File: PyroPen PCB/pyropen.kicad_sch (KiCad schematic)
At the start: 58 parts, among them J1 AAAA BATT, J2 Front 3.3v LED, J3 MLX90614ESF-DCC-000-TU, J4 BUZZ, J5 DEBUG, SW1 B3U-1000P, U1 ATTINY1616-MNR, U2 MAX17222ELT+T

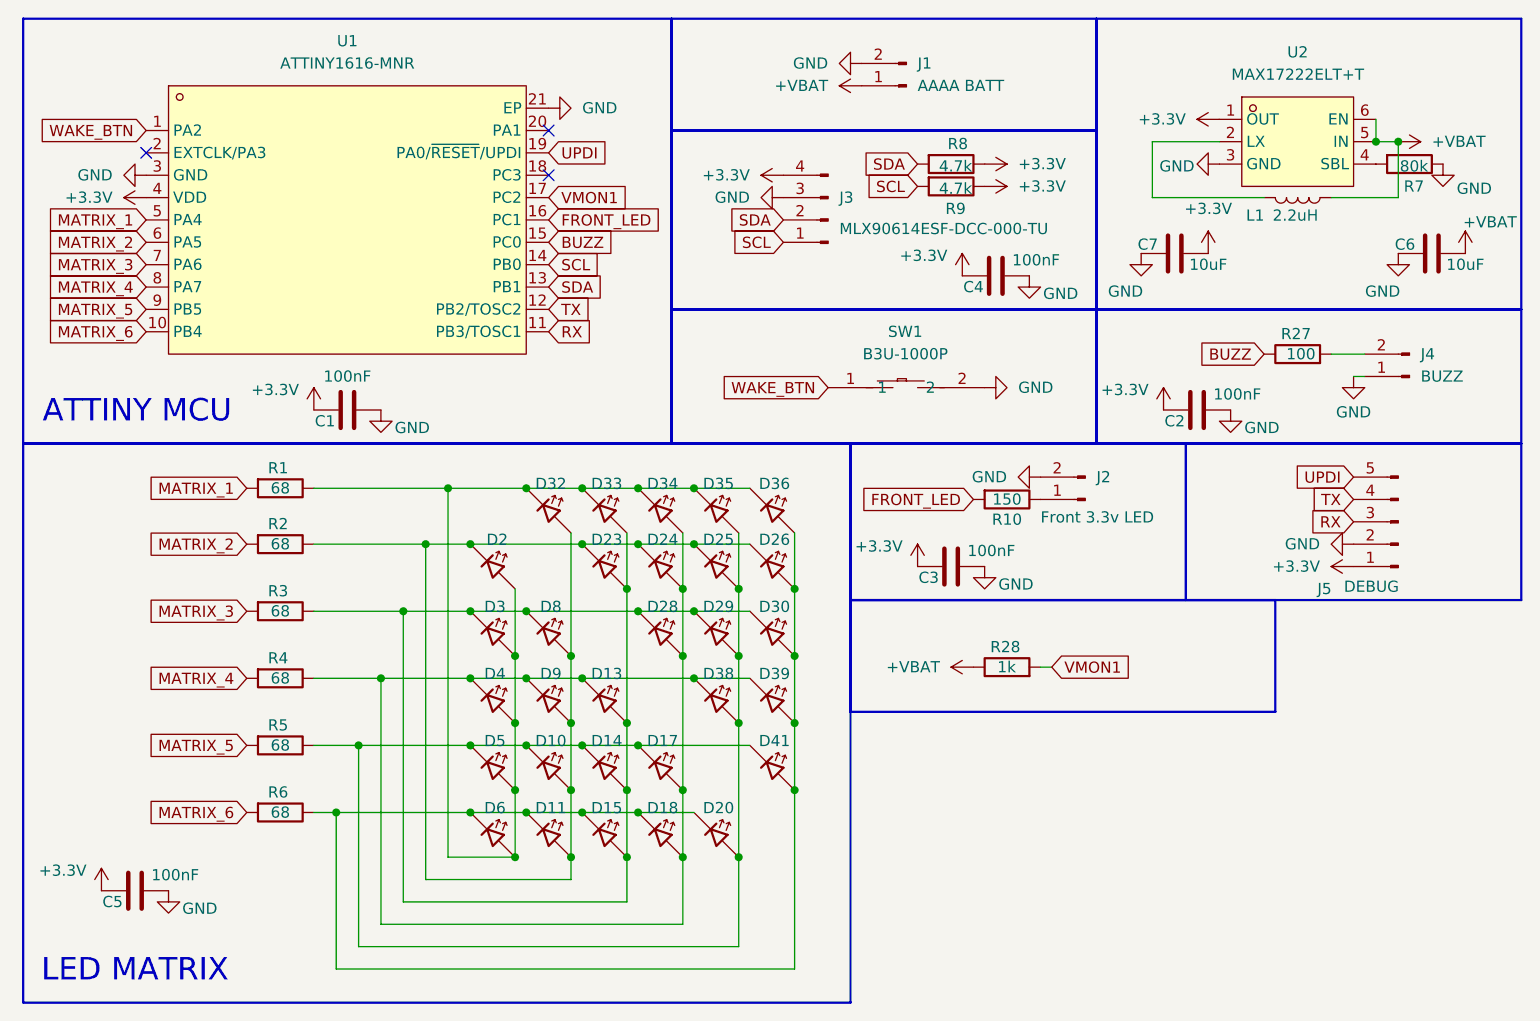
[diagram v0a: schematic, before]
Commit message: sync
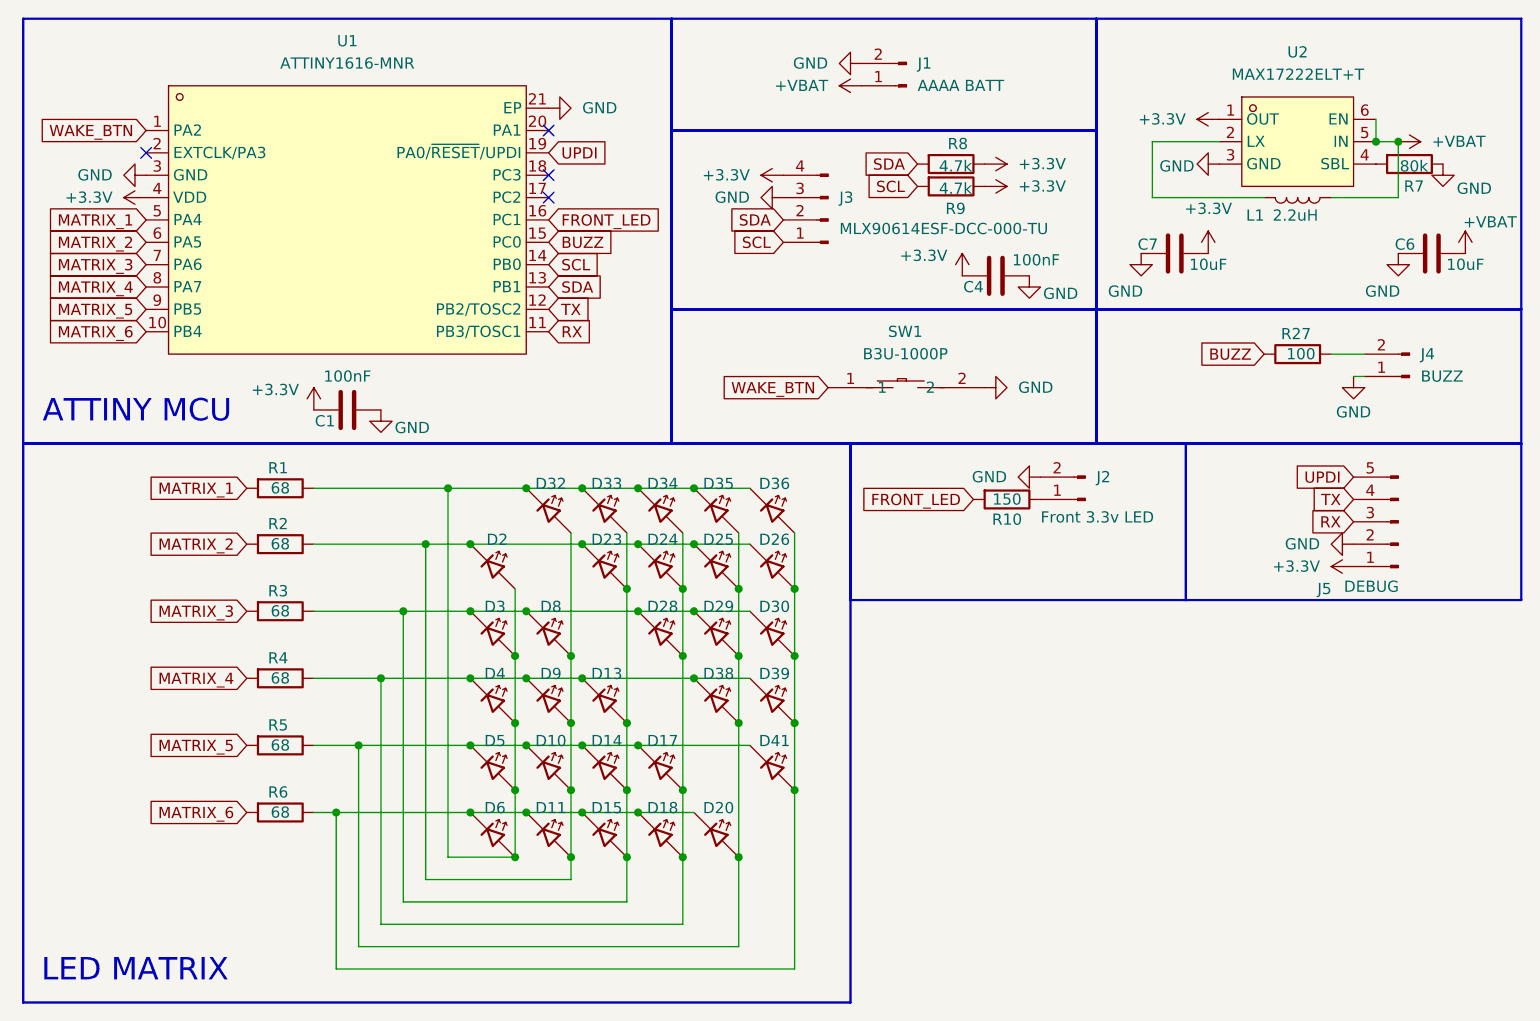
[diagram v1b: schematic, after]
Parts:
- removed C2, C3, C5: 100nF, Capacitor_SMD:C_0402_1005Metric, symbol Device:C
- removed R28: 1k, Resistor_SMD:R_0402_1005Metric, symbol Device:R
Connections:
- net VMON1: no longer names the net of U1.17 (PC2)
- no-connect marks 3 -> 4

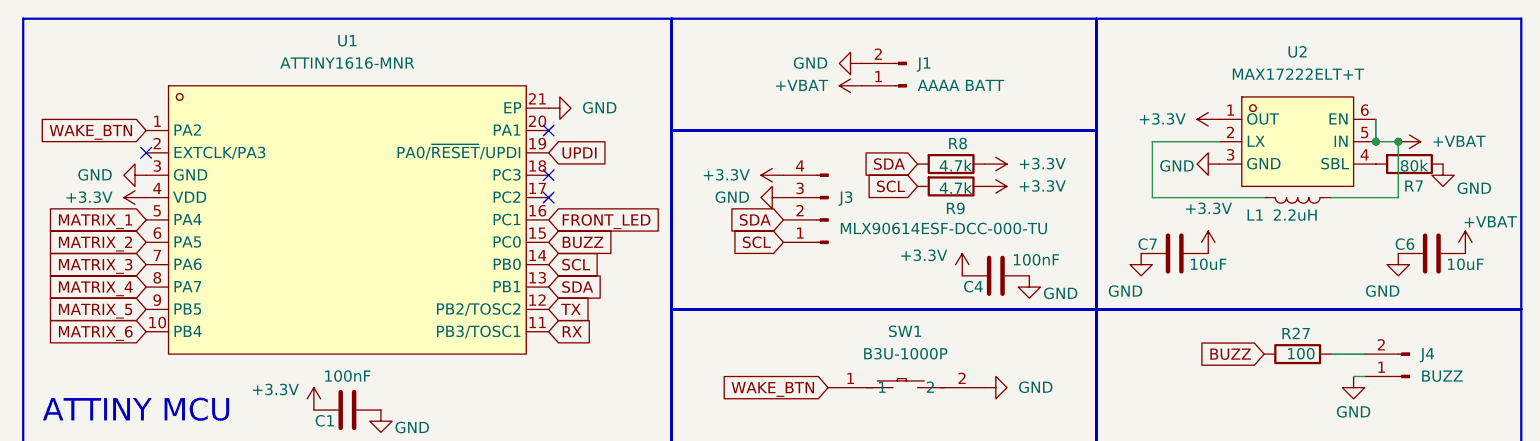
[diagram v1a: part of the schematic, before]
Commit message: sync
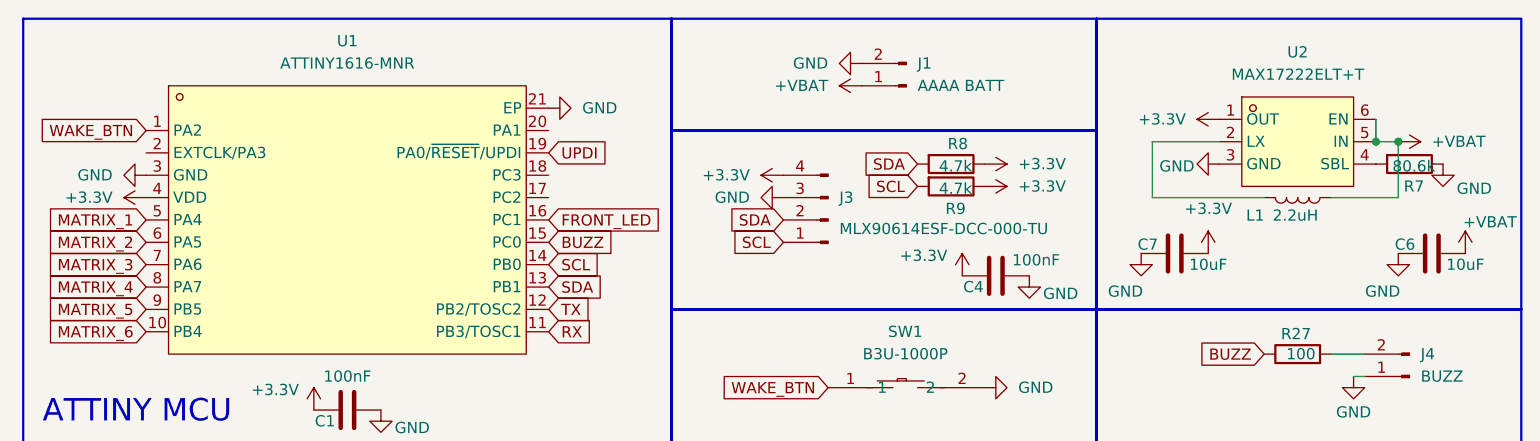
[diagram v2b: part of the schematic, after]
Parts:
- R7: value 80k -> 80.6k
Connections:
- no-connect marks 4 -> 0
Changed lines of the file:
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@@
 		(color 0 0 0 0)
 	)
-	(no_connect
-		(at 74.93 30.48)
-	)
-	(no_connect
-		(at 74.93 25.4)
-	)
-	(no_connect
-		(at 29.21 27.94)
-	)
-	(no_connect
-		(at 74.93 33.02)
-	)
 	(wire
 		(pts
@@
 			)
 		)
-		(property "Value" "80k"
+		(property "Value" "80.6k"
 			(at 173.228 29.464 90)
 			(show_name no)

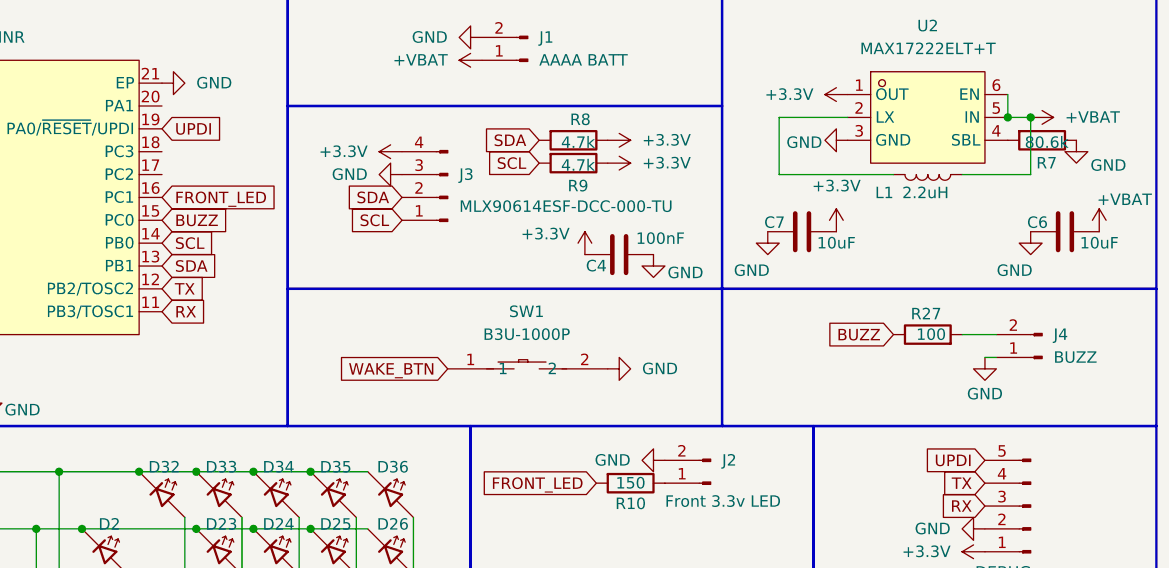
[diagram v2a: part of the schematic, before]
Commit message: sync
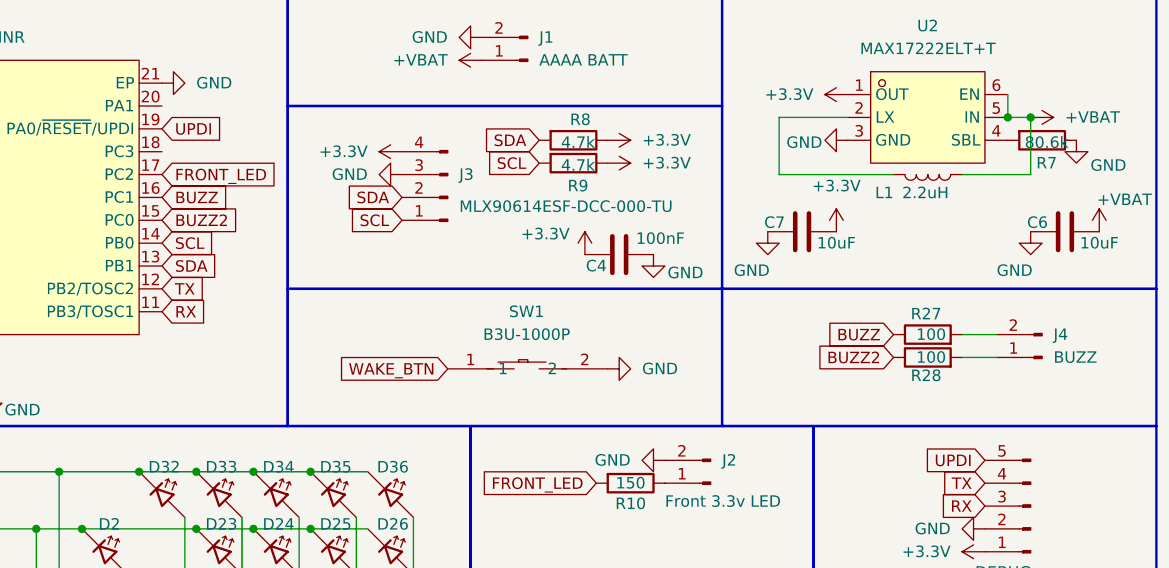
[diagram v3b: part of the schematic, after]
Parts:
- added R28: 100, Resistor_SMD:R_0402_1005Metric, symbol Device:R
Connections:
- net BUZZ: now also U1.16 (PC1); no longer U1.15 (PC0)
- net FRONT_LED: now also U1.17 (PC2); no longer U1.16 (PC1)
- net GND: no longer J4.1 (Pin_1)
- new net: J4.1 (Pin_1), R28.2
- new net BUZZ2: R28.1, U1.15 (PC0)
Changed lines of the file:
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@@
 	(wire
 		(pts
-			(xy 166.37 53.34) (xy 167.64 53.34)
-		)
-		(stroke
-			(width 0)
-			(type default)
-		)
-	)
-	(wire
-		(pts
 			(xy 66.04 80.01) (xy 72.39 80.01)
 		)
@@
 	(wire
 		(pts
+			(xy 163.83 53.34) (xy 167.64 53.34)
+		)
+		(stroke
+			(width 0)
+			(type default)
+		)
+	)
+	(wire
+		(pts
 			(xy 50.8 102.87) (xy 50.8 120.65)
 		)
@@
 		)
 	)
+	(global_label "BUZZ2"
+		(shape input)
+		(at 156.21 53.34 180)
+		(fields_autoplaced yes)
+		(effects
+			(font
+				(size 1.27 1.27)
+			)
+			(justify right)
+		)
+		(property "Intersheetrefs" "${INTERSHEET_REFS}"
+			(at 146.9958 53.34 0)
+			(hide yes)
+			(show_name no)
+			(do_not_autoplace no)
+			(effects
+				(font
+					(size 1.27 1.27)
+				)
+				(justify right)
+			)
+		)
+	)
 	(global_label "TX"
 		(shape input)
@@
 		)
 	)
-	(global_label "BUZZ"
+	(global_label "BUZZ2"
 		(shape input)
 		(at 74.93 38.1 0)
@@
 		)
 		(property "Intersheetrefs" "${INTERSHEET_REFS}"
-			(at 82.9347 38.1 0)
+			(at 84.1442 38.1 0)
 			(hide yes)
 			(show_name no)
@@
 		)
 	)
+	(global_label "BUZZ"
+		(shape input)
+		(at 74.93 35.56 0)
+		(fields_autoplaced yes)
+		(effects
+			(font
+				(size 1.27 1.27)
+			)
+			(justify left)
+		)
+		(property "Intersheetrefs" "${INTERSHEET_REFS}"
+			(at 82.9347 35.56 0)
+			(hide yes)
+			(show_name no)
+			(do_not_autoplace no)
+			(effects
+				(font
+					(size 1.27 1.27)
+				)
+				(justify left)
+			)
+		)
+	)
 	(global_label "SDA"
 		(shape input)
@@
 	(global_label "FRONT_LED"
 		(shape input)
-		(at 74.93 35.56 0)
+		(at 74.93 33.02 0)
 		(fields_autoplaced yes)
 		(effects
@@
 		)
 		(property "Intersheetrefs" "${INTERSHEET_REFS}"
-			(at 88.3171 35.56 0)
+			(at 88.3171 33.02 0)
 			(hide yes)
 			(show_name no)
@@
 	)
 	(symbol
+		(lib_id "Device:R")
+		(at 160.02 53.34 90)
+		(unit 1)
+		(body_style 1)
+		(exclude_from_sim no)
+		(in_bom yes)
+		(on_board yes)
+		(in_pos_files yes)
+		(dnp no)
+		(property "Reference" "R28"
+			(at 161.544 55.372 90)
+			(show_name no)
+			(do_not_autoplace no)
+			(effects
+				(font
+					(size 1.27 1.27)
+				)
+				(justify left)
+			)
+		)
+		(property "Value" "100"
+			(at 162.052 53.34 90)
+			(show_name no)
+			(do_not_autoplace no)
+			(effects
+				(font
+					(size 1.27 1.27)
+				)
+				(justify left)
+			)
+		)
+		(property "Footprint" "Resistor_SMD:R_0402_1005Metric"
+			(at 160.02 55.118 90)
+			(hide yes)
+			(show_name no)
+			(do_not_autoplace no)
+			(effects
+				(font
+					(size 1.27 1.27)
+				)
+			)
+		)
+		(property "Datasheet" ""
+			(at 160.02 53.34 0)
+			(hide yes)
+			(show_name no)
+			(do_not_autoplace no)
+			(effects
+				(font
+					(size 1.27 1.27)
+				)
+			)
+		)
+		(property "Description" "Resistor"
+			(at 160.02 53.34 0)
+			(hide yes)
+			(show_name no)
+			(do_not_autoplace no)
+			(effects
+				(font
+					(size 1.27 1.27)
+				)
+			)
+		)
+		(pin "2"
+		)
+		(pin "1"
+		)
+		(instances
+			(project "pyropen"
+				(path "/3064dcfd-3f6b-4110-b282-8b370e19b43b"
+					(reference "R28")
+					(unit 1)
+				)
+			)
+		)
+	)
+	(symbol
 		(lib_id "Device:LED_45deg")
 		(at 93.98 82.55 180)
@@
 					(unit 1)
 				)
-			)
-		)
-	)
-	(symbol
-		(lib_id "power:GND")
-		(at 166.37 53.34 0)
-		(unit 1)
-		(body_style 1)
-		(exclude_from_sim no)
-		(in_bom yes)
-		(on_board yes)
-		(in_pos_files yes)
-		(dnp no)
-		(property "Reference" "#PWR0102"
-			(at 166.37 59.69 0)
-			(hide yes)
-			(show_name no)
-			(do_not_autoplace no)
-			(effects
-				(font
-					(size 1.27 1.27)
-				)
-			)
-		)
-		(property "Value" "GND"
-			(at 166.37 57.404 0)
-			(show_name no)
-			(do_not_autoplace no)
-			(effects
-				(font
-					(size 1.27 1.27)
-				)
-			)
-		)
-		(property "Footprint" ""
-			(at 166.37 53.34 0)
-			(hide yes)
-			(show_name no)
-			(do_not_autoplace no)
-			(effects
-				(font
-					(size 1.27 1.27)
-				)
-			)
-		)
-		(property "Datasheet" ""
-			(at 166.37 53.34 0)
-			(hide yes)
-			(show_name no)
-			(do_not_autoplace no)
-			(effects
-				(font
-					(size 1.27 1.27)
-				)
-			)
-		)
-		(property "Description" "Power symbol creates a global label with name \"GND\" , ground"
-			(at 166.37 53.34 0)
-			(hide yes)
-			(show_name no)
-			(do_not_autoplace no)
-			(effects
-				(font
-					(size 1.27 1.27)
-				)
-			)
-		)
-		(pin "1"
-		)
-		(instances
-			(project "pyropen"
-				(path "/3064dcfd-3f6b-4110-b282-8b370e19b43b"
-					(reference "#PWR0102")
-					(unit 1)
-				)
